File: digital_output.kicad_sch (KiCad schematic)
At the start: 16 parts, among them Q1 AOSP21321, Q2 AOSP21321, Q3 DMN2056U, Q4 DMN2056U

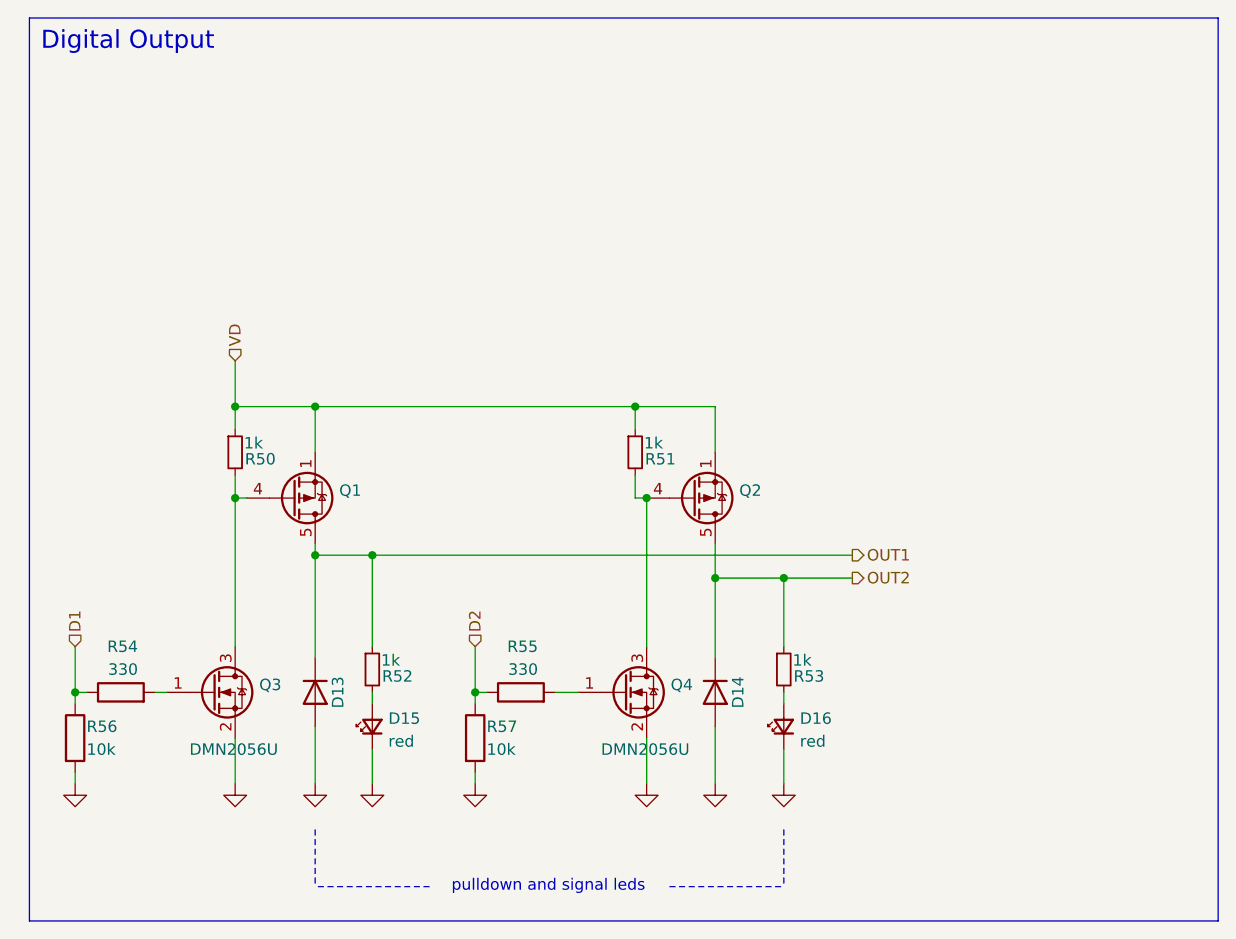
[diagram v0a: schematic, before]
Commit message: started routing
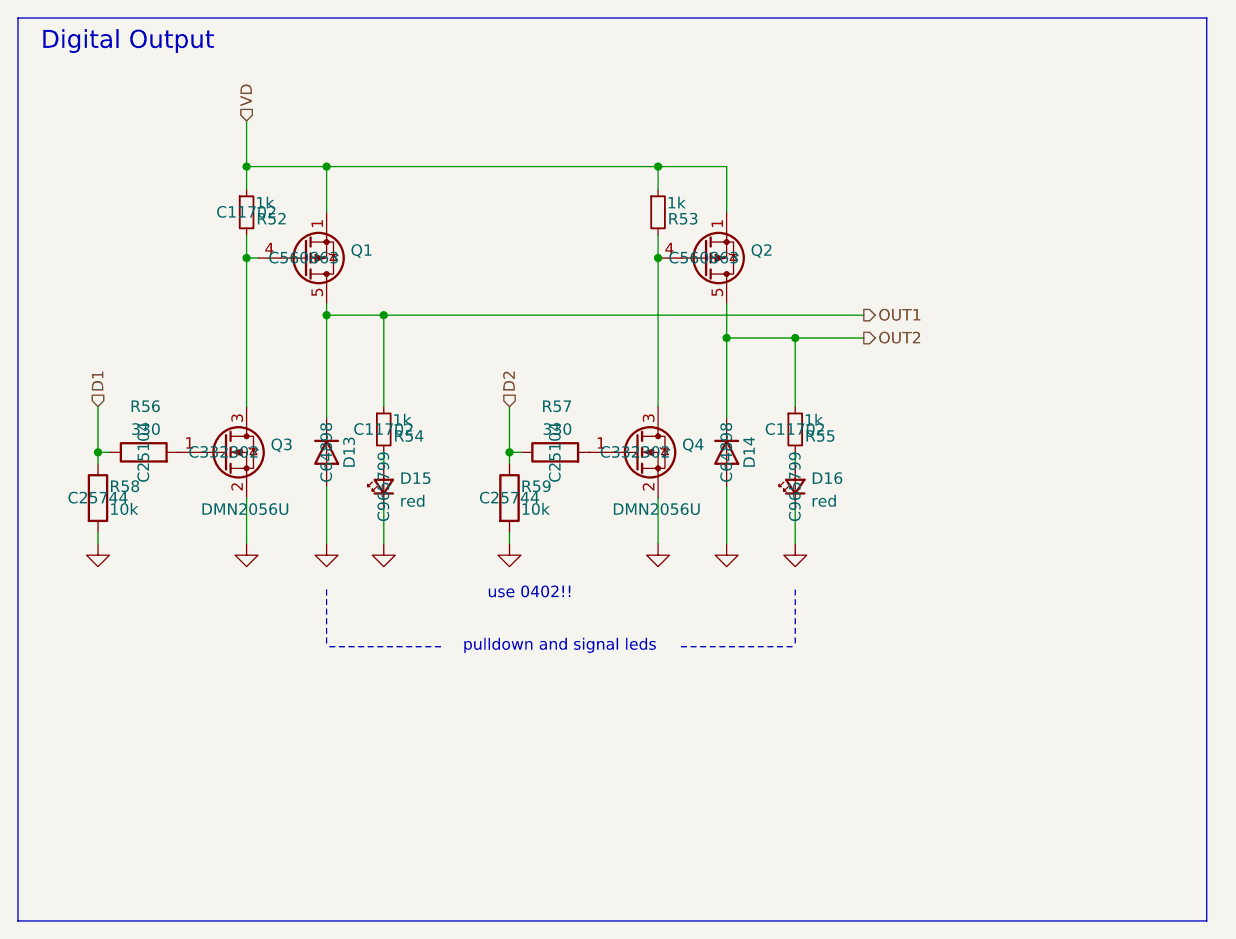
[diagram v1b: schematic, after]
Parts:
- D13, D14: footprint Diode_SMD:D_SOD-323_HandSoldering -> Diode_SMD:D_SOD-123F; LCSC (none) -> C64898; LCSC# C7528872 -> (none)
- D15, D16: LCSC (none) -> C965799; LCSC# C965799 -> (none)
- Q1, Q2: footprint Package_SO:SO-8_3.9x4.9mm_P1.27mm -> Package_SO:SOIC-8_3.9x4.9mm_P1.27mm; LCSC (none) -> C560863; LCSC# C560863 -> (none)
- R52: renamed from R50; LCSC (none) -> C11702; LCSC# C2906899 -> (none); Manufacturer FOJAN -> (none); Part# FRC0402J102 TS -> (none)
- R53: renamed from R51; LCSC (none) -> C11702; LCSC# C2906899 -> (none); Manufacturer FOJAN -> (none); Part# FRC0402J102 TS -> (none)
- R54: renamed from R52; LCSC (none) -> C11702; LCSC# C2906899 -> (none); Manufacturer FOJAN -> (none); Part# FRC0402J102 TS -> (none)
- R55: renamed from R53; LCSC (none) -> C11702; LCSC# C2906899 -> (none); Manufacturer FOJAN -> (none); Part# FRC0402J102 TS -> (none)
- R56: renamed from R54; footprint Resistor_SMD:R_0603_1608Metric_Pad0.98x0.95mm_HandSolder -> Resistor_SMD:R_0402_1005Metric; LCSC (none) -> C25104; LCSC# C23138 -> (none)
- R57: renamed from R55; footprint Resistor_SMD:R_0603_1608Metric_Pad0.98x0.95mm_HandSolder -> Resistor_SMD:R_0402_1005Metric; LCSC (none) -> C25104; LCSC# C23138 -> (none)
- R58: renamed from R56; footprint Resistor_SMD:R_0603_1608Metric_Pad0.98x0.95mm_HandSolder -> Resistor_SMD:R_0402_1005Metric; LCSC (none) -> C25744; LCSC# C25804 -> (none)
- R59: renamed from R57; footprint Resistor_SMD:R_0603_1608Metric_Pad0.98x0.95mm_HandSolder -> Resistor_SMD:R_0402_1005Metric; LCSC (none) -> C25744; LCSC# C25804 -> (none)
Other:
- note added: "use 0402!!"
- moved on the sheet: D13, D14, D15, D16, Q1, Q2, Q3, Q4, R52, R53, R54, R55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

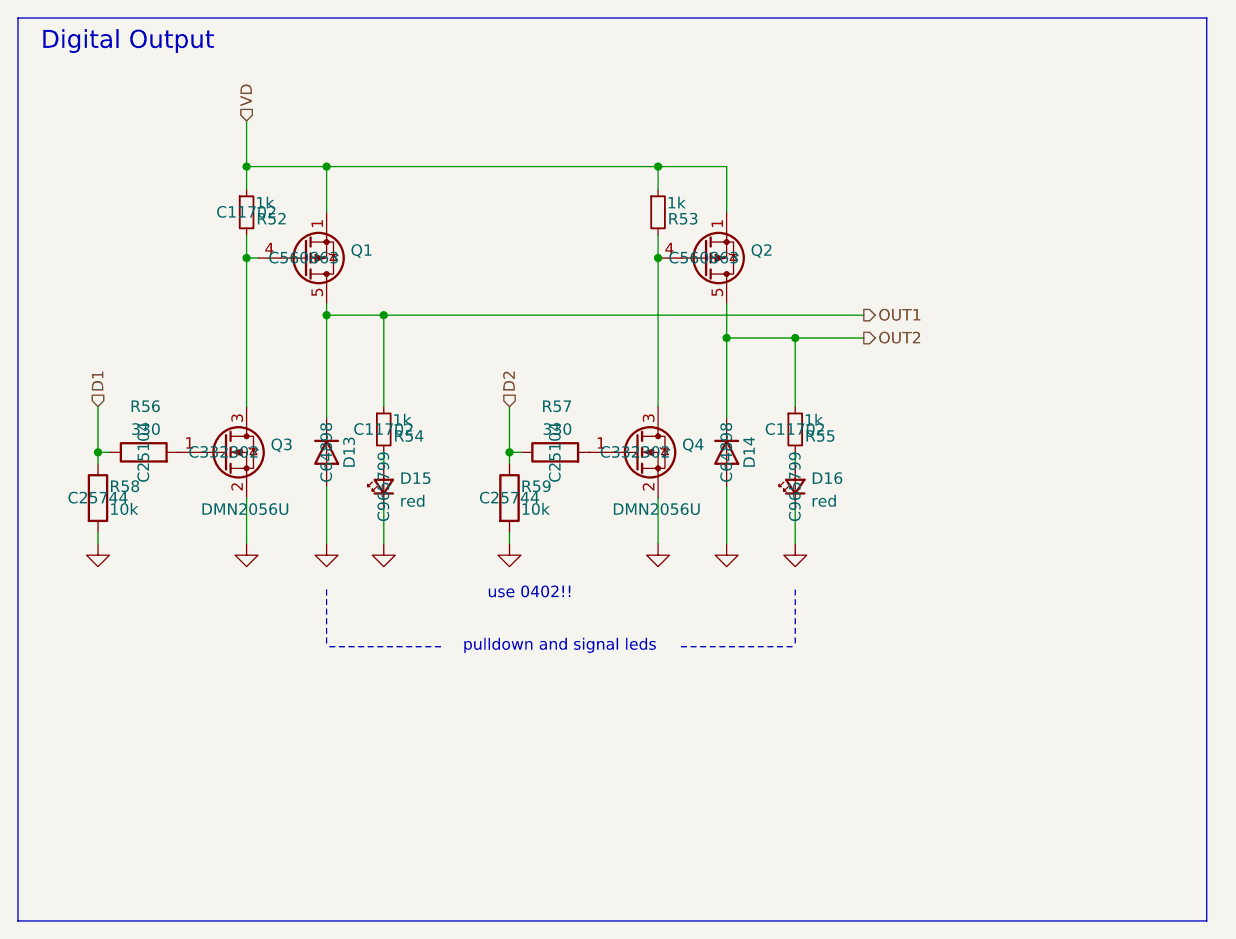
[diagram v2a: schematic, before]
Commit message: finished routing
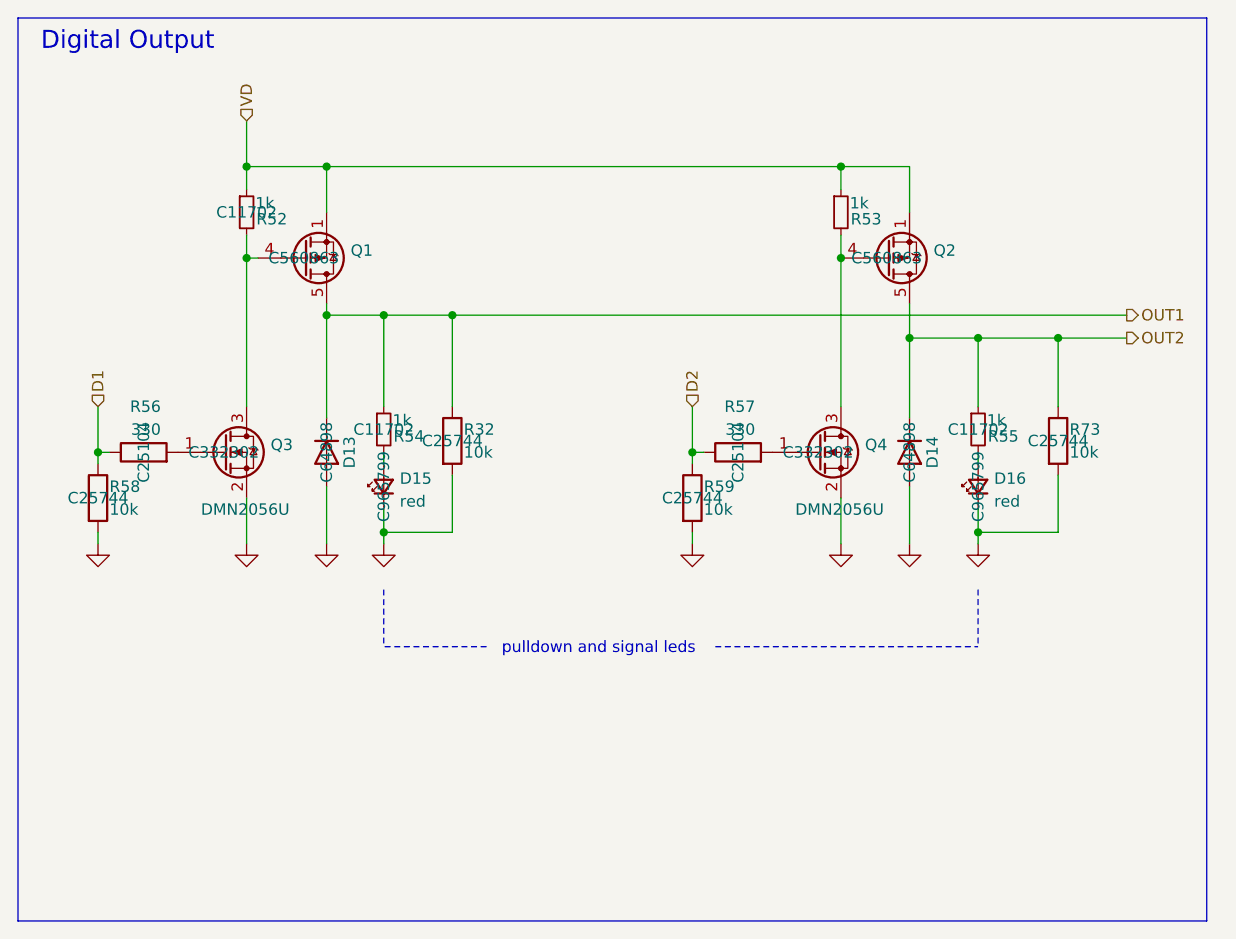
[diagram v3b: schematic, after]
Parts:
- added R32, R73: 10k, Resistor_SMD:R_0402_1005Metric, symbol Device:R
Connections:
- net GND: now also R32.2, R73.2
- net OUT1: now also R32.1
- net OUT2: now also R73.1
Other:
- note removed: "use 0402!!"
- moved on the sheet: D14, D16, Q2, Q4, R53, R55, R57, R59

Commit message: started silkscrean
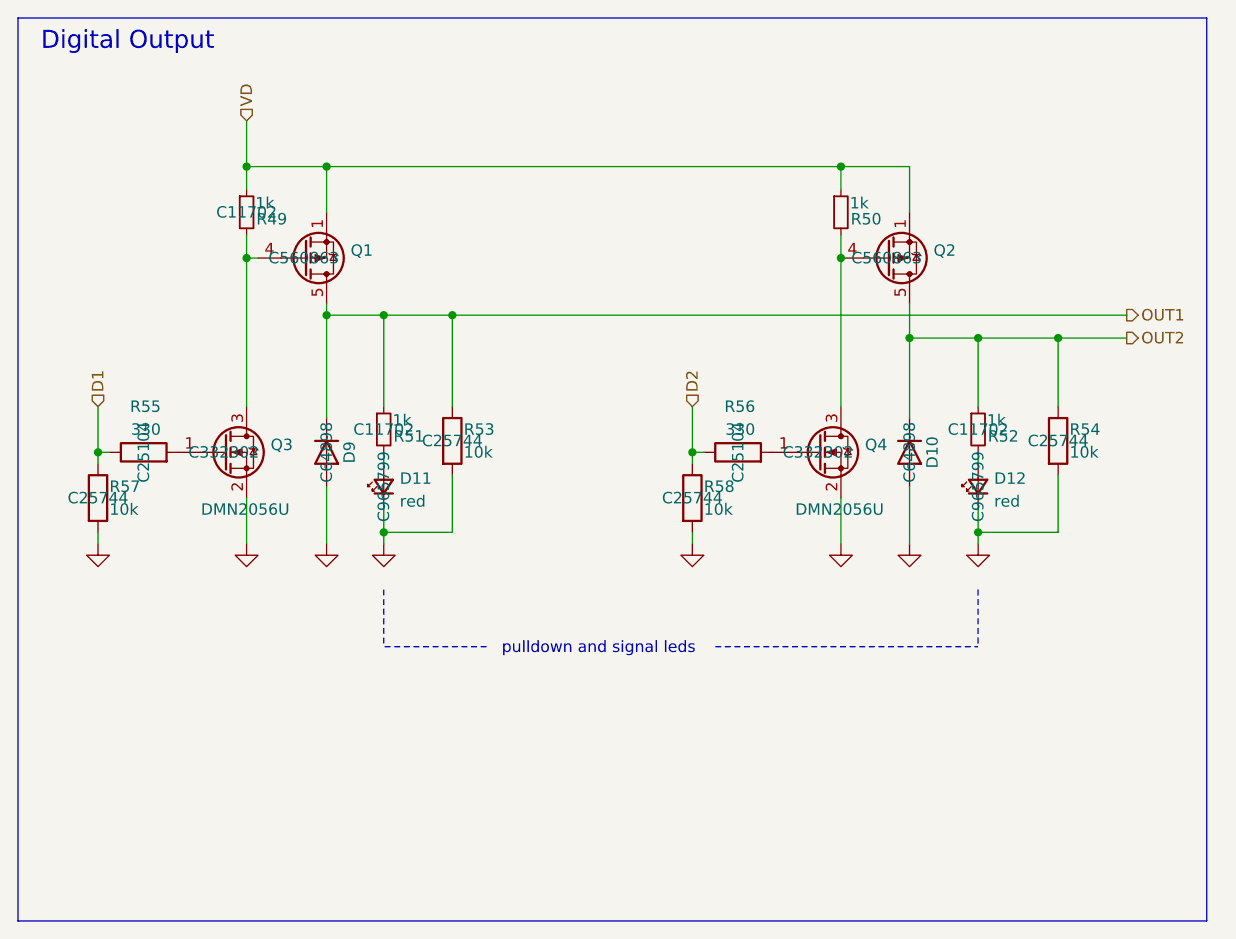
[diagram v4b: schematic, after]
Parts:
- renumbered D14 to D10, D15 to D11, D16 to D12, D13 to D9, R52 to R49, R53 to R50, R54 to R51, R55 to R52, R32 to R53, R73 to R54, R56 to R55, R57 to R56, R58 to R57, R59 to R58
